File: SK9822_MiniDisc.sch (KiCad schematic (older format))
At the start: 369 parts, among them P1 CONN_01X04, P2 CONN_01X04

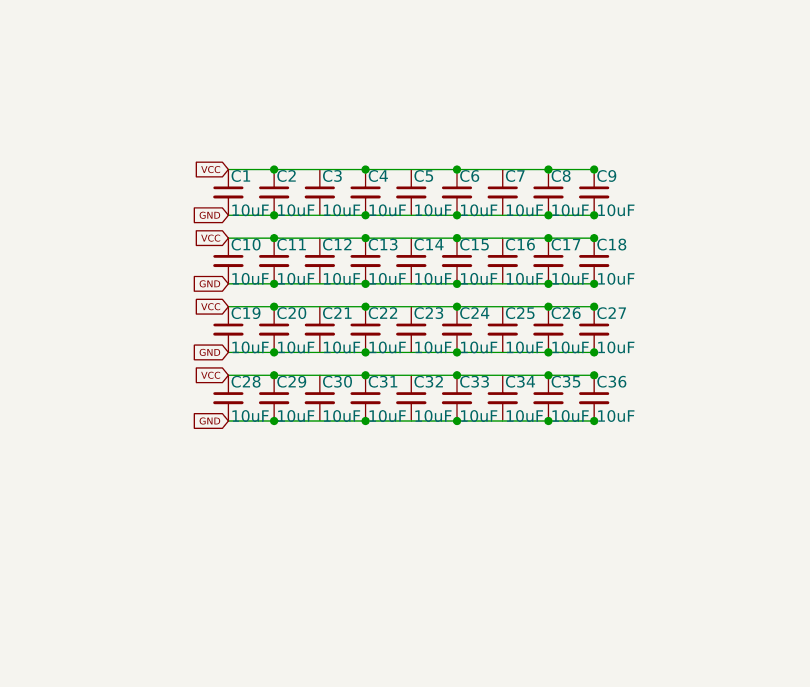
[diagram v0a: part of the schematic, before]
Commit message: finaly got caps right
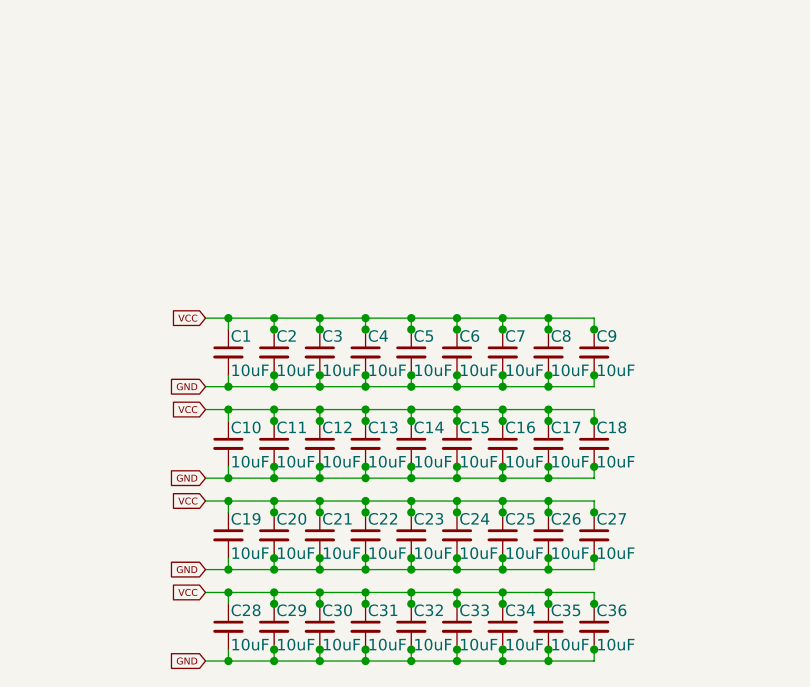
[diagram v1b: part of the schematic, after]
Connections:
- net GND: now also C12.2, C14.2, C16.2, C21.2, C23.2, C25.2, C3.2, C30.2, C32.2, C34.2, C5.2, C7.2
- net VCC: now also C12.1, C14.1, C16.1, C21.1, C23.1, C25.1, C3.1, C30.1, C32.1, C34.1, C5.1, C7.1
